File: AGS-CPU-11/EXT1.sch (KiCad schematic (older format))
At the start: 9 parts, among them P5 EXT1

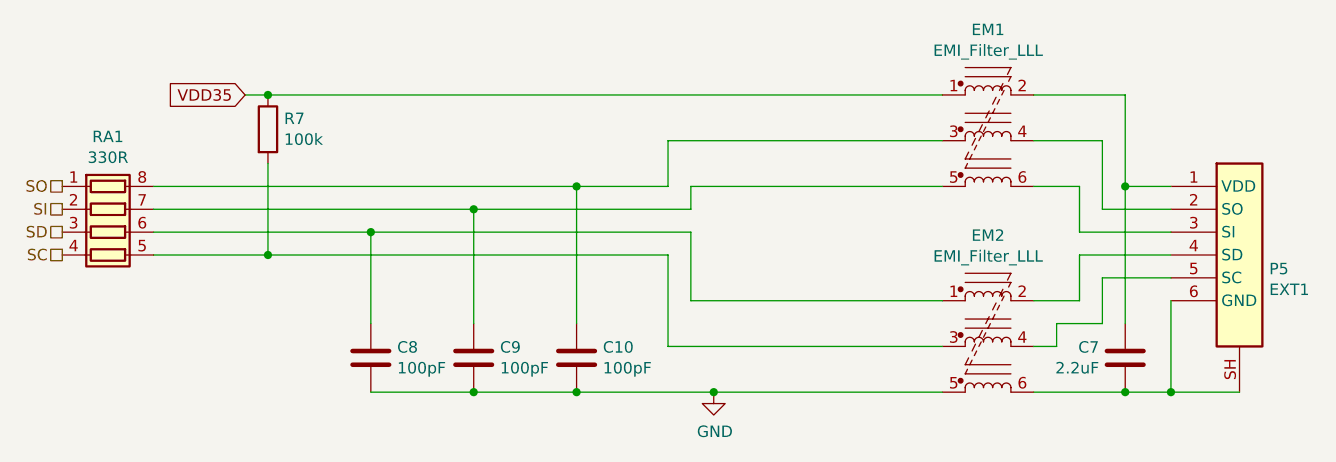
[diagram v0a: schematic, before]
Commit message: Fix location of pull-up resistor R7
Fixes #2
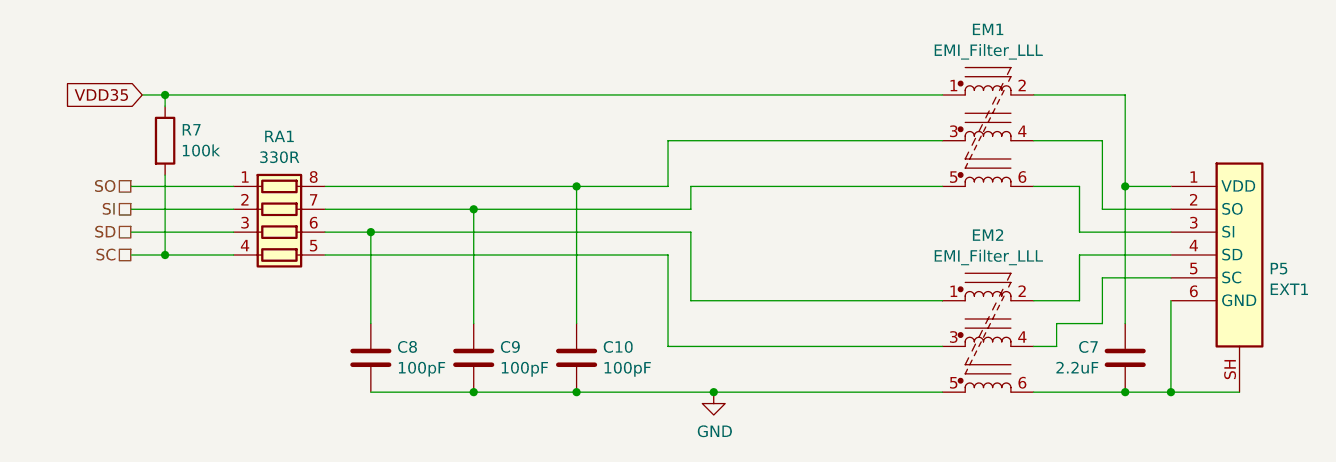
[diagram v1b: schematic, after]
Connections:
- net SC: now also R7.2
- net at EM2.3, RA1.5 (R4.2): no longer R7.2
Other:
- moved on the sheet: R7, RA1
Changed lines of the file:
@@
 L Device:R_Pack04 RA?
 U 1 1 5BD74727
-P 2750 3700
+P 3500 3700
 AR Path="/5BD74727" Ref="RA?"  Part="1"
 AR Path="/5BD73A5E/5BD74727" Ref="RA1"  Part="1"
-F 0 "RA1" V 2333 3700 50  0000 C CNN
-F 1 "330R" V 2424 3700 50  0000 C CNN
-F 2 "" V 3025 3700 50  0001 C CNN
-F 3 "~" H 2750 3700 50  0001 C CNN
-	1    2750 3700
+F 0 "RA1" V 3083 3700 50  0000 C CNN
+F 1 "330R" V 3174 3700 50  0000 C CNN
+F 2 "" V 3775 3700 50  0001 C CNN
+F 3 "~" H 3500 3700 50  0001 C CNN
+	1    3500 3700
 	0    1    1    0
 $EndComp
@@
 $EndComp
 Wire Wire Line
-	2950 3500 4800 3500
+	3700 3500 4800 3500
 Wire Wire Line
 	4800 3500 4800 4100
 Wire Wire Line
-	2950 3600 4350 3600
-Wire Wire Line
-	2950 3700 3900 3700
-Wire Wire Line
-	2950 3800 3450 3800
+	3700 3600 4350 3600
+Wire Wire Line
+	3700 3700 3900 3700
 Connection ~ 4800 3500
 Wire Wire Line
@@
 	4800 4400 5400 4400
 Connection ~ 4800 4400
-Text GLabel 3350 3100 0    50   Input ~ 0
+Text GLabel 2900 3100 0    50   Input ~ 0
 VDD35
-Text HLabel 2550 3500 0    50   UnSpc ~ 0
+Text HLabel 2850 3500 0    50   UnSpc ~ 0
 SO
-Text HLabel 2550 3600 0    50   UnSpc ~ 0
+Text HLabel 2850 3600 0    50   UnSpc ~ 0
 SI
-Text HLabel 2550 3700 0    50   UnSpc ~ 0
+Text HLabel 2850 3700 0    50   UnSpc ~ 0
 SD
-Text HLabel 2550 3800 0    50   UnSpc ~ 0
+Text HLabel 2850 3800 0    50   UnSpc ~ 0
 SC
 Wire Wire Line
@@
 	5300 3500 6400 3500
 Wire Wire Line
-	3350 3100 3450 3100
+	2900 3100 3000 3100
 Wire Wire Line
 	6400 3300 5200 3300
@@
 L Device:R R?
 U 1 1 61574D8A
-P 3450 3250
+P 3000 3300
 AR Path="/61574D8A" Ref="R?"  Part="1"
 AR Path="/5BD73A5E/61574D8A" Ref="R7"  Part="1"
-F 0 "R7" H 3520 3296 50  0000 L CNN
-F 1 "100k" H 3520 3205 50  0000 L CNN
-F 2 "" V 3380 3250 50  0001 C CNN
-F 3 "~" H 3450 3250 50  0001 C CNN
-	1    3450 3250
-	1    0    0    -1
-$EndComp
-Connection ~ 3450 3100
-Wire Wire Line
-	3450 3100 6400 3100
-Wire Wire Line
-	3450 3400 3450 3800
-Connection ~ 3450 3800
-Wire Wire Line
-	3450 3800 5200 3800
+F 0 "R7" H 3070 3346 50  0000 L CNN
+F 1 "100k" H 3070 3255 50  0000 L CNN
+F 2 "" V 2930 3300 50  0001 C CNN
+F 3 "~" H 3000 3300 50  0001 C CNN
+	1    3000 3300
+	1    0    0    -1
+$EndComp
+Connection ~ 3000 3100
+Wire Wire Line
+	3000 3100 6400 3100
 $Comp
 L Device:C C?
@@
 	1    0    0    -1
 $EndComp
+Wire Wire Line
+	3700 3800 5200 3800
+Wire Wire Line
+	2850 3800 3000 3800
+Wire Wire Line
+	3000 3800 3000 3450
+Connection ~ 3000 3800
+Wire Wire Line
+	3000 3800 3300 3800
+Wire Wire Line
+	2850 3500 3300 3500
+Wire Wire Line
+	2850 3600 3300 3600
+Wire Wire Line
+	2850 3700 3300 3700
+Wire Wire Line
+	3000 3150 3000 3100
 $EndSCHEMATC
